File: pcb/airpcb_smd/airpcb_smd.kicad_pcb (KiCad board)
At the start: 2 copper layers, 49 x 65 mm, 26 parts, among them J1 I2C, J11 PSU, J2 DHT, J3 DC, J4 AB, J7 PWR, J8 WS2812, J9 5V3V, Q1 PN2222A, Q2 PN2222A, U1 PC817, U2 PC817, U3 ESP32-DEVKIT-V1

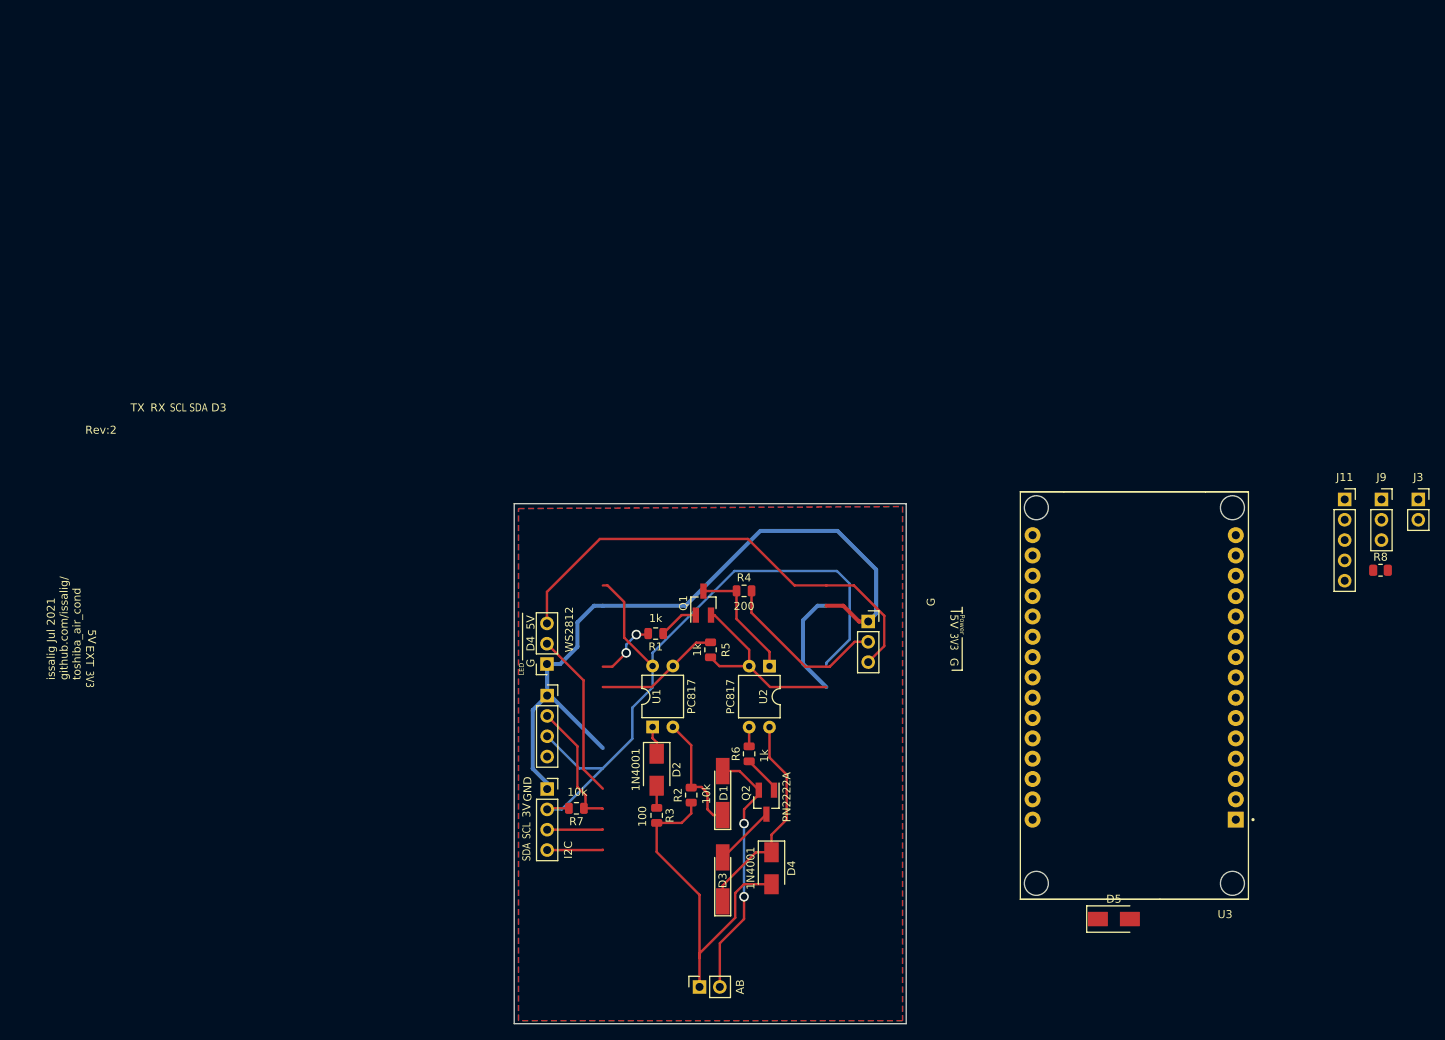
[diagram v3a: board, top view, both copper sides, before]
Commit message: pcb wip
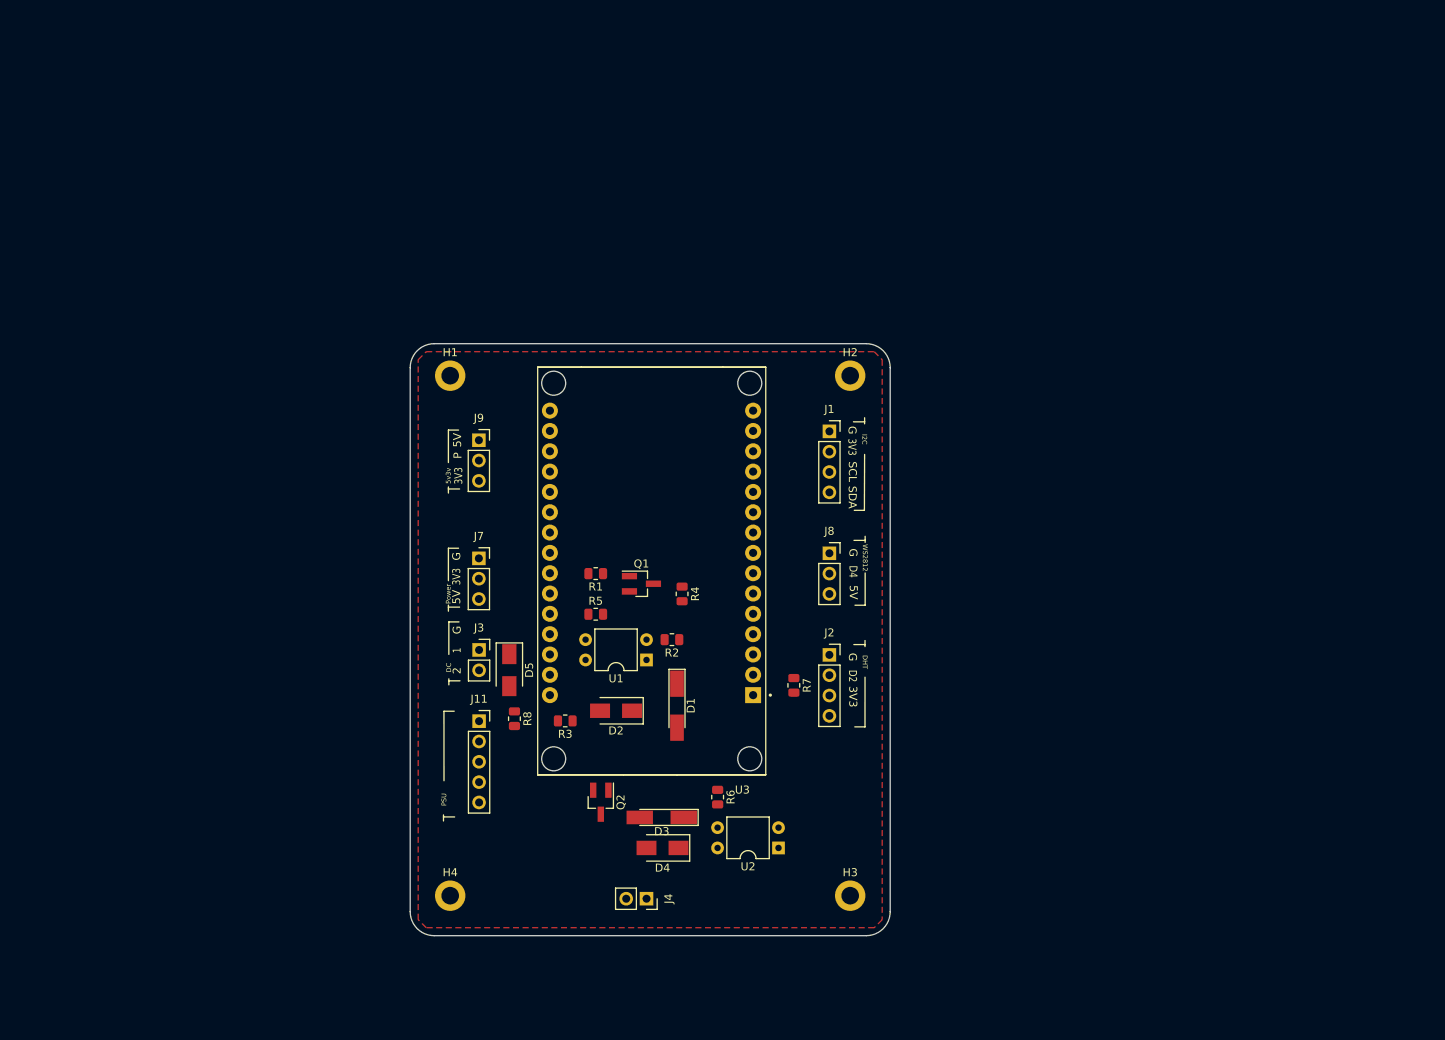
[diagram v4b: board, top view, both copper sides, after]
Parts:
- added H1: MountingHole, MountingHole:MountingHole_2.2mm_M2_DIN965_Pad, F.Cu at (105.0, 54.0)
- added H2: MountingHole, MountingHole:MountingHole_2.2mm_M2_DIN965_Pad, F.Cu at (155.0, 54.0)
- added H3: MountingHole, MountingHole:MountingHole_2.2mm_M2_DIN965_Pad, F.Cu at (155.0, 119.0)
- added H4: MountingHole, MountingHole:MountingHole_2.2mm_M2_DIN965_Pad, F.Cu at (105.0, 119.0)
- moved J3 118.9 mm to (108.6, 88.3)
- moved J9 113.1 mm to (108.6, 62.1)
- moved J11 111.7 mm to (108.6, 97.2)
- moved R8 109.8 mm to (113.0, 96.9), turned to -90 degrees
- moved D5 81.7 mm to (112.4, 90.8), turned to -90 degrees
- moved U3 62.3 mm to (130.2, 78.4)
- moved J1 57.0 mm to (152.4, 61.0)
- moved J7 49.3 mm to (108.6, 76.8)
- moved J8 37.9 mm to (152.4, 76.2), turned to 0 degrees
- moved J2 35.6 mm to (152.4, 88.9)
- moved R7 31.2 mm to (148.0, 92.7), turned to -90 degrees
- moved U2 22.8 mm to (146.0, 113.0), turned to 180 degrees
- moved Q2 20.7 mm to (123.8, 107.3)
- moved R2 19.6 mm to (132.7, 87.0), turned to 180 degrees
- moved R3 16.4 mm to (119.4, 97.2), turned to 180 degrees
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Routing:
- net GND: track 129.4 -> 0.00 mm
- net 3V3: track 113.0 -> 0.00 mm
- net 5V: track 59.4 -> 0.00 mm
- net A: track 43.8 -> 0.00 mm
- net B: track 32.1 -> 0.00 mm, vias 2 -> 0
- net Net-(D3-Pad1): track 27.1 -> 0.00 mm
- net D4: track 21.0 -> 0.00 mm
- net D2: track 16.0 -> 0.00 mm
- net D12: track 15.8 -> 0.00 mm
- net Net-(Q1-Pad3): track 15.3 -> 0.00 mm
- net Net-(D1-Pad1): track 15.1 -> 0.00 mm
- net D13: track 7.98 -> 0.00 mm, vias 2 -> 0
- net Net-(D3-Pad2): track 7.70 -> 0.00 mm
- net SCL: track 6.98 -> 0.00 mm
- net SDA: track 6.98 -> 0.00 mm
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- added copper zone on F.Cu, net GND
- removed copper zone on B.Cu, net 3V3
- removed copper zone on F.Cu, net 3V3
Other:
- board size 49 x 65 mm -> 60 x 74 mm
- board text added: "1"
- board text added: "2"
- board text added: "5v3v"
- board text added: "D2"
- board text added: "DC"
- board text added: "DHT"
- board text added: "I2C"
- board text added: "P"
- board text added: "PSU"
- board text added: "WS2812"
- board text removed: "3V"
- board text removed: "D3"
- board text removed: "EXT"
- board text removed: "GND"
- board text removed: "LED"
- board text removed: "RX"
- board text removed: "Rev:2"
- board text removed: "TX"
- board text removed: "issalig Jul 2021 github.com/issalig/ toshiba_air_cond"
